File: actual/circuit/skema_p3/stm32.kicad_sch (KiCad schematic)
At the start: 36 parts, among them J2 Conn_01x05_Male, J3 USB_B_Micro, J4 Micro_SD_Card_Det_Hirose_DM3AT, SW6 SW_Push, SW7 SW_Push, SW8 SW_Push, SW9 SW_Push, U3 STM32F303RBTx

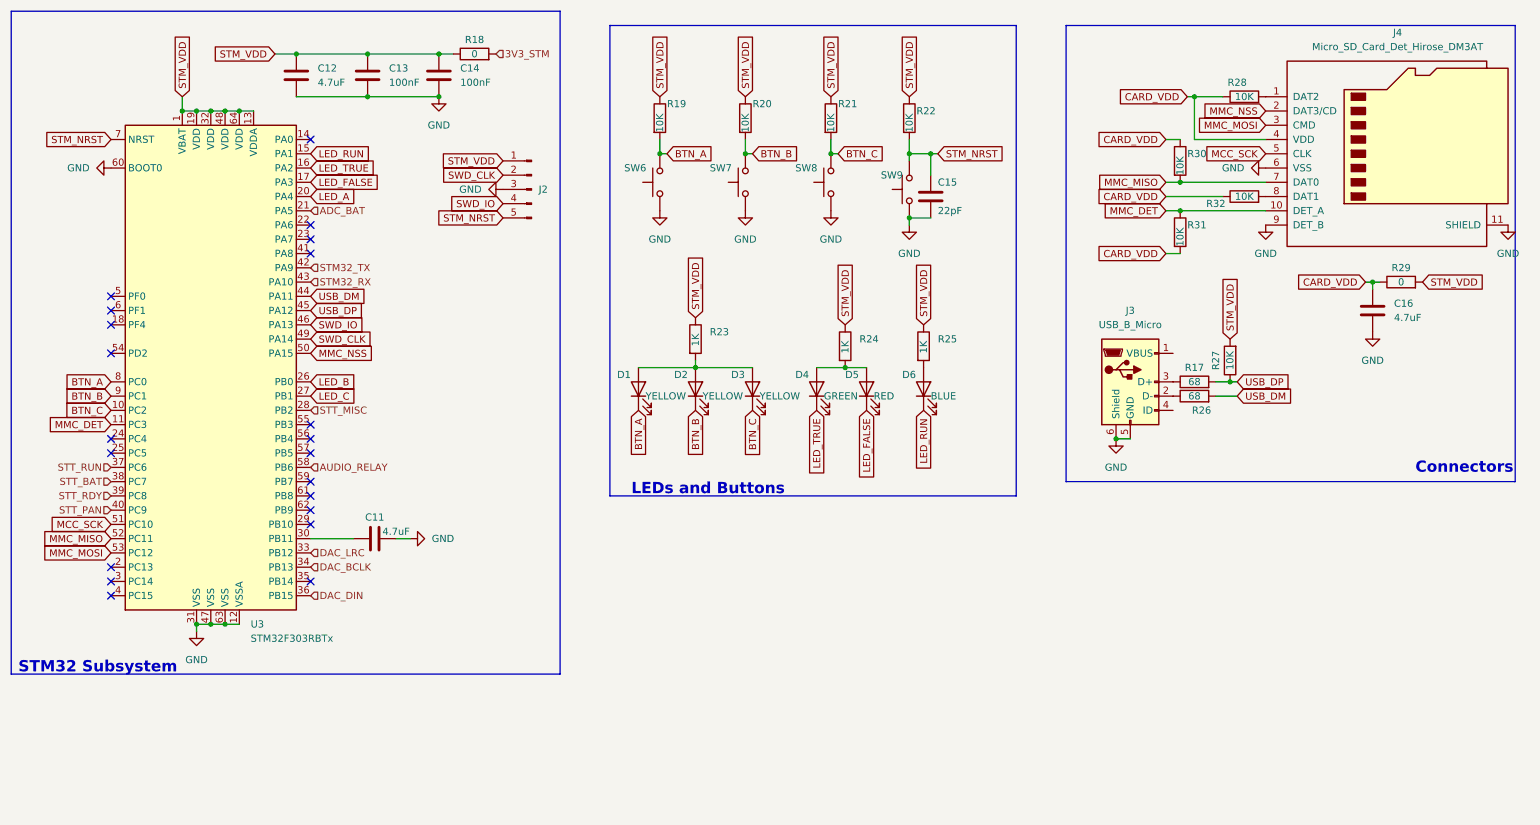
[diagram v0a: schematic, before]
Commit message: P3 in KiCAD
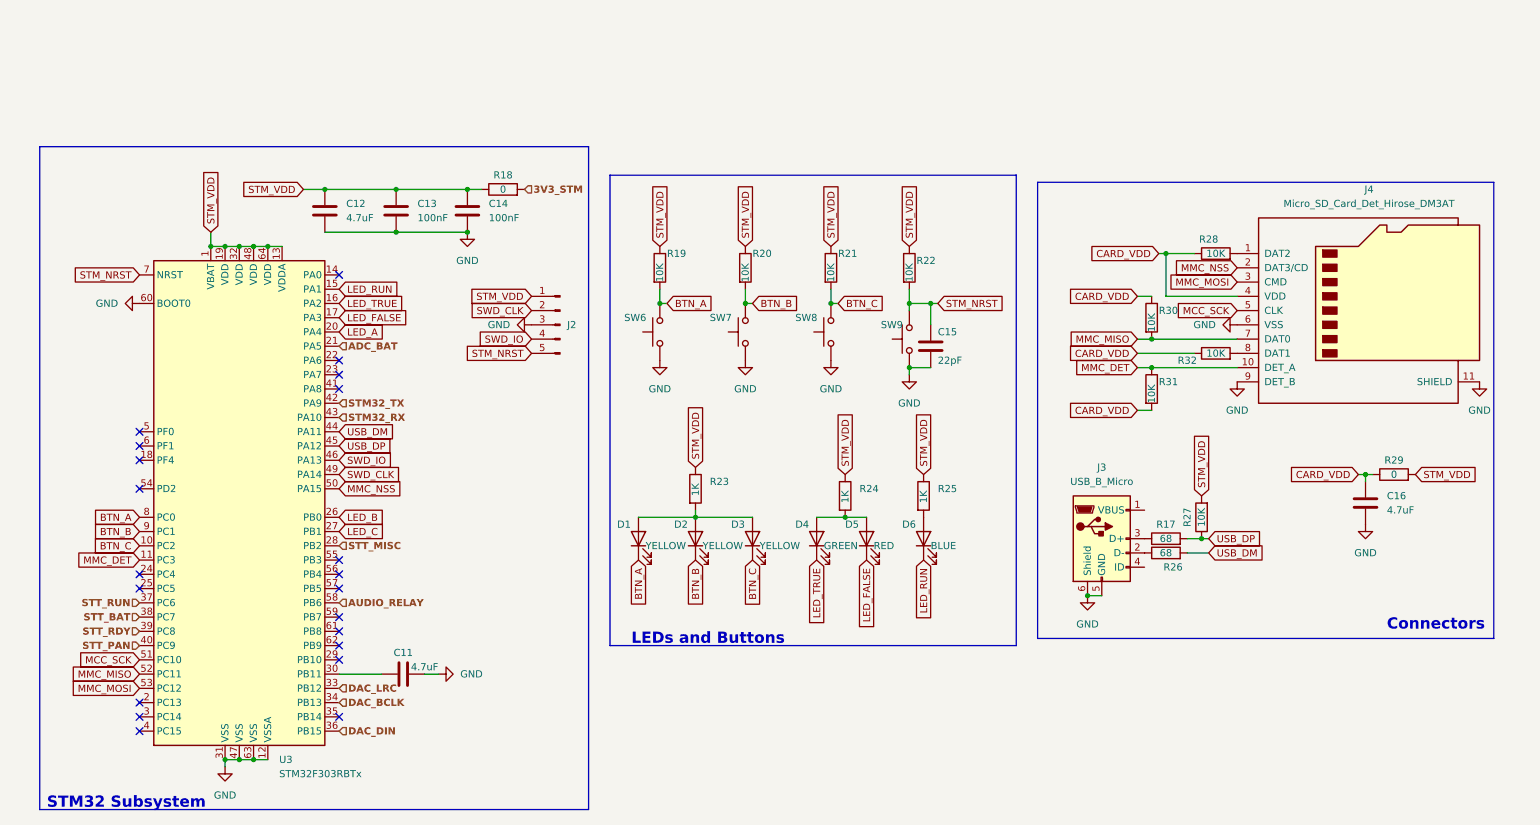
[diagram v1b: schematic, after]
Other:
- moved on the sheet: C11, C12, C13, C14, C15, C16, D1, D2, D3, D4, D5, D6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
